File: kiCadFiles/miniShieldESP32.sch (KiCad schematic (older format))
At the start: 38 parts, among them J1 VIM, J2 OUT, J3 I2C, J4 I2C, J5 I2C, Q1 BC846, Q2 BC846, Q3 BC846, Q4 BC846, Q5 BC846, SW1 SW_Push, SW2 SW_Push, SW3 SP6T, U1 ESP32-DEVKITC-32D, U2 DHT11, U3 L7805

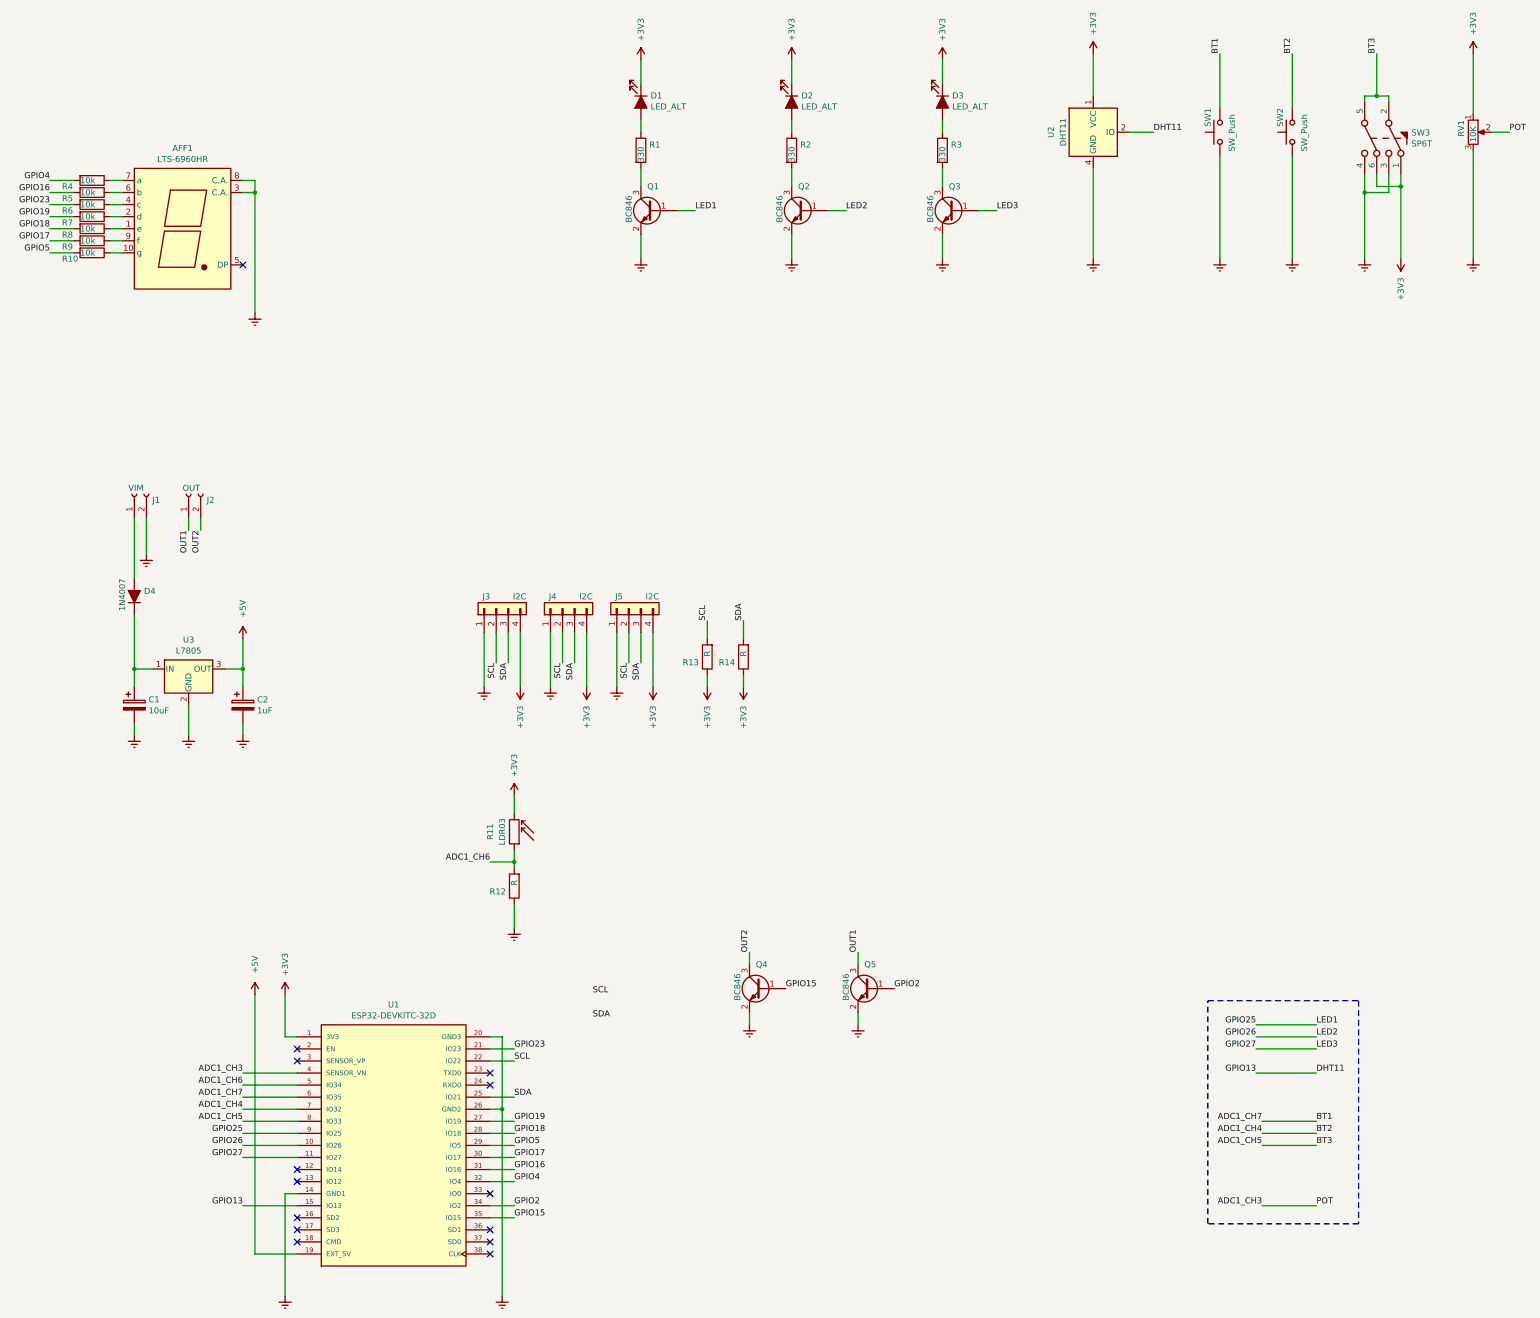
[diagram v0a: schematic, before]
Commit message: update
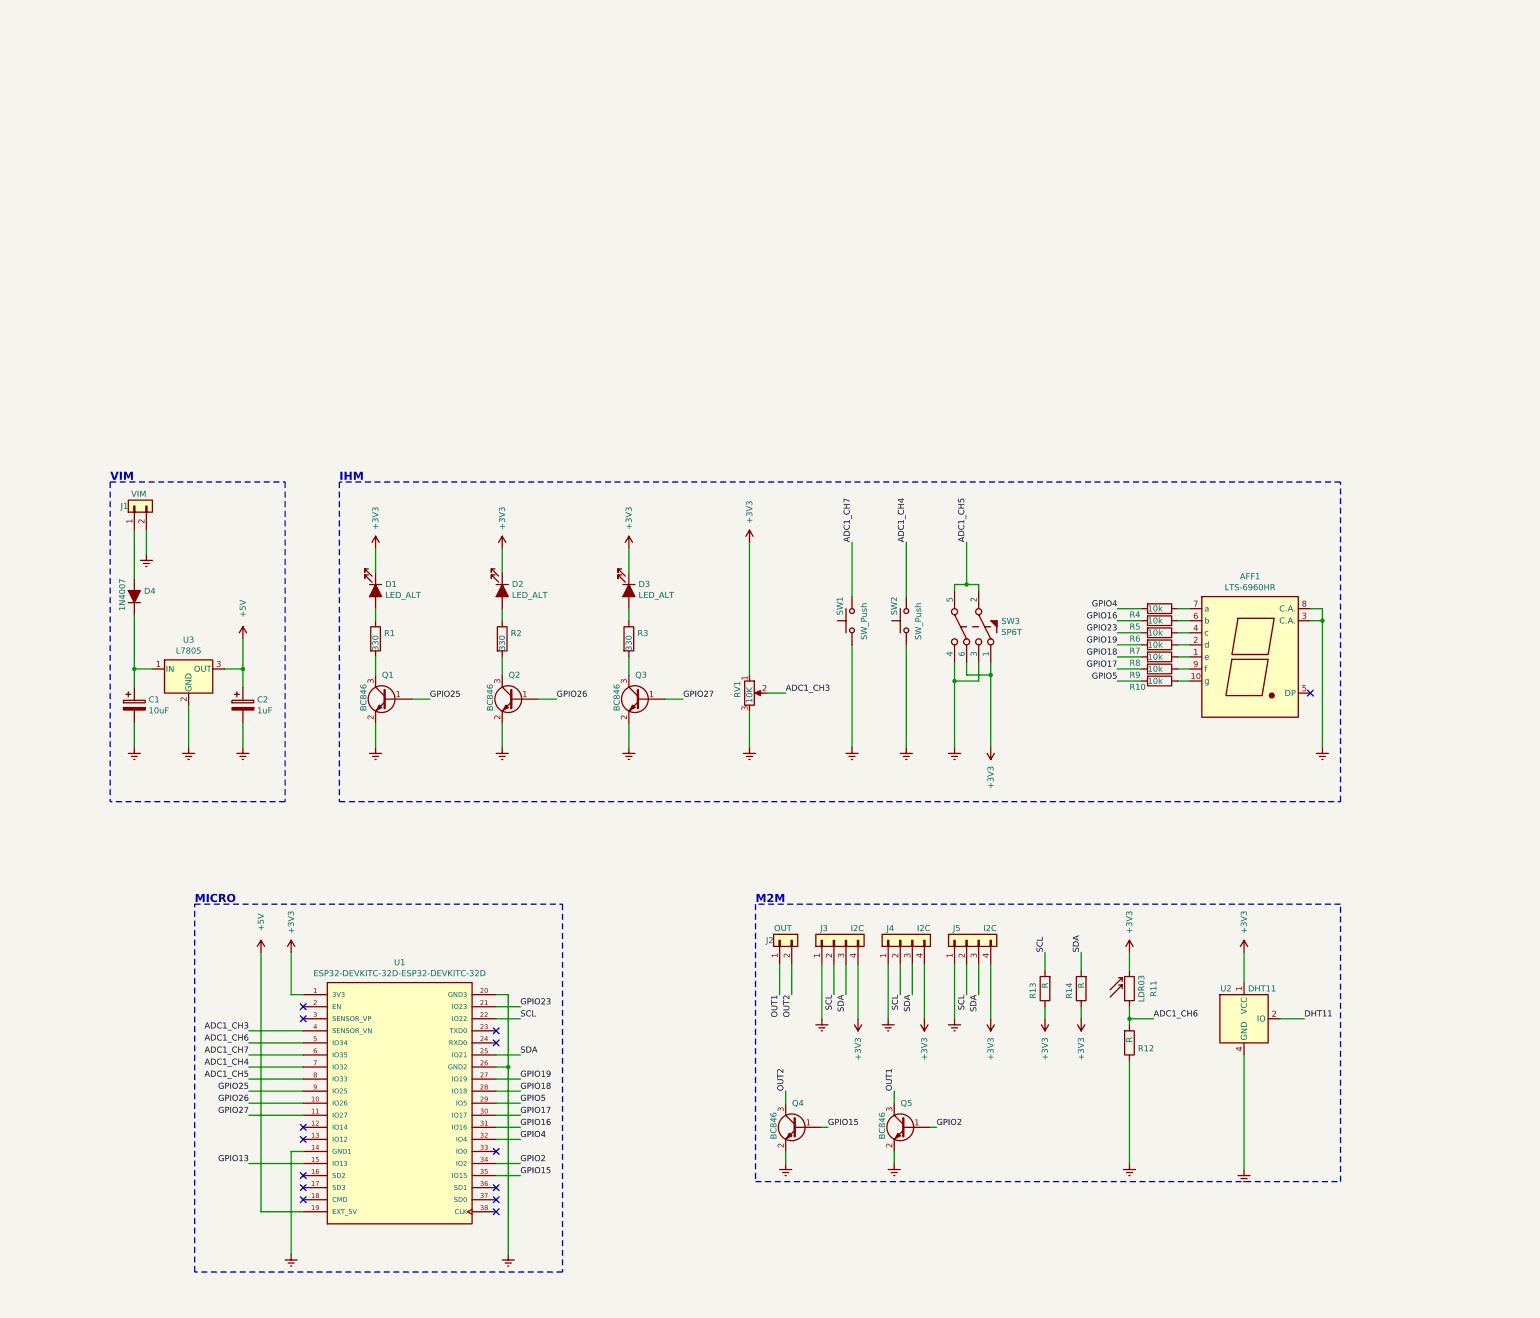
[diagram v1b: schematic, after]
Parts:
- removed J1: VIM, MyFootprint:AK300-2, symbol Connector:Conn_01x02_Female
- removed J2: OUT, MyFootprint:AK300-2, symbol Connector:Conn_01x02_Female
- removed U1: ESP32-DEVKITC-32D, MyFootprint:MODULE_ESP32-DEVKITC-32D, symbol ESP32-DEVKITC-32D:ESP32-DEVKITC-32D
- added J1: VIM, MyFootprint:AK300-2, symbol Connector_Generic:Conn_01x02
- added J2: OUT, MyFootprint:AK300-2, symbol Connector_Generic:Conn_01x02
- added U1: ESP32-DEVKITC-32D-ESP32-DEVKITC-32D, MODULE_ESP32-DEVKITC-32D, symbol miniShieldESP32-rescue:ESP32-DEVKITC-32D-ESP32-DEVKITC-32D
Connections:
- net +3V3: now also U1.1 (3V3)
- net +5V: now also U1.19 (EXT_5V)
- net ADC1_CH3: now also U1.4 (SENSOR_VN)
- net ADC1_CH4: now also U1.7 (IO32)
- net ADC1_CH5: now also U1.8 (IO33)
- net ADC1_CH6: now also U1.5 (IO34)
- net ADC1_CH7: now also U1.6 (IO35)
- net Earth: now also J1.2 (Pin_2), U1.14 (GND1), U1.20 (GND3), U1.26 (GND2)
- net GPIO15: now also U1.35 (IO15)
- net GPIO16: now also U1.31 (IO16)
- net GPIO17: now also U1.30 (IO17)
- net GPIO18: now also U1.28 (IO18)
- net GPIO19: now also U1.27 (IO19)
- net GPIO2: now also U1.34 (IO2)
- net GPIO23: now also U1.21 (IO23)
- net GPIO25: now also U1.9 (IO25)
- net GPIO26: now also U1.10 (IO26)
- net GPIO27: now also U1.11 (IO27)
- net GPIO4: now also U1.32 (IO4)
- net GPIO5: now also U1.29 (IO5)
- net OUT1: now also J2.1 (Pin_1)
- net OUT2: now also J2.2 (Pin_2)
- net SCL: now also U1.22 (IO22)
- net SDA: now also U1.25 (IO21)
- net at D4.2 (A): now also J1.1 (Pin_1)
- new net GPIO13: U1.15 (IO13)
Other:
- note added: "IHM"
- note added: "M2M"
- note added: "MICRO"
- note added: "VIM"
- moved on the sheet: AFF1, D1, D2, D3, J3, J4, J5, Q1, Q2, Q3, Q4, Q5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
